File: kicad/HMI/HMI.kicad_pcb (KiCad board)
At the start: 2 copper layers, 45 parts, among them J2 SWD, J3 DEM 128128A TMH-PW-N, J4 RIBBON, SW1 SW_Push, SW10 SW_Push, SW11 SW_Push, SW12 SW_Push, SW13 SW_Push, SW14 SW_Push, SW15 SW_Push, SW16 SW_Push, SW17 SW_Push, SW18 SW_Push, SW19 SW_Push, SW2 SW_Push, SW20 SW_Push, SW3 SW_Push, SW4 SW_Push, SW5 SW_Push, SW6 SW_Push, SW7 SW_Push, SW8 SW_Push, SW9 SW_Push, U1 STM32L011K4Tx, X1 ASV-4.000MHZ-EJ-T

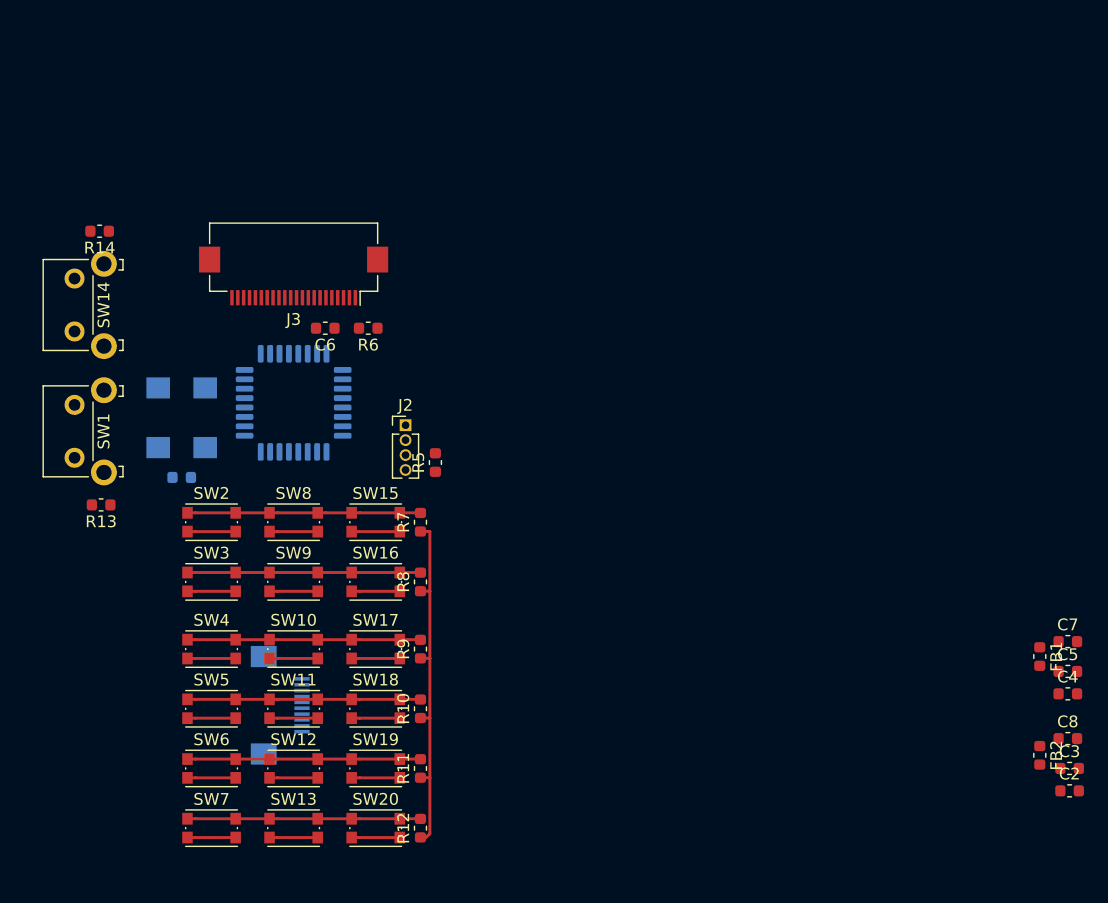
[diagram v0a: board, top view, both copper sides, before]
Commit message: HMI: added design of PCB -> plotted PDF -> plotted production output - Gerbers -> HMI is READY!!
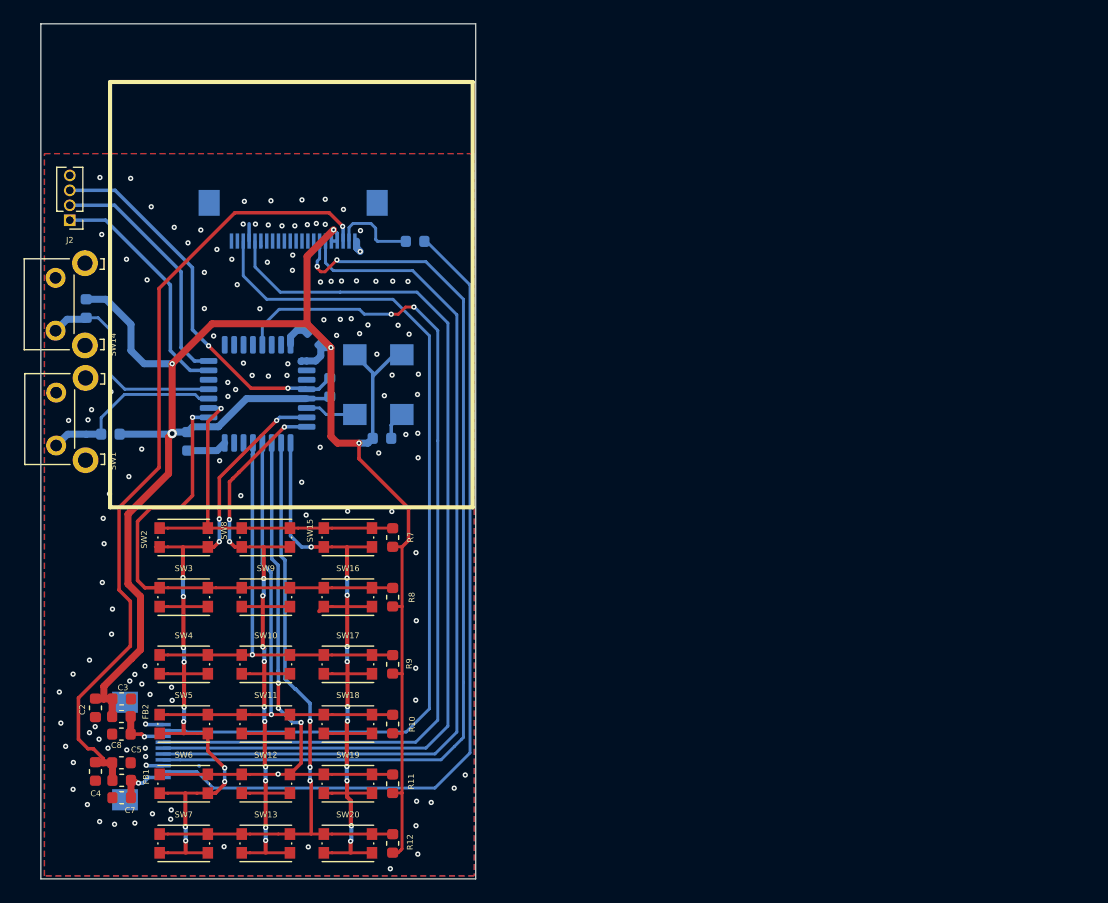
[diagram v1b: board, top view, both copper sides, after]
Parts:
- added C9: 1u, Capacitor_SMD:C_0603_1608Metric, B.Cu at (93.8, 67.5)
- C6, J3, R13, R14, R5, R6: moved to B.Cu
- moved C2 83.2 mm to (75.2, 99.0), turned to 270 degrees
- moved C4 83.0 mm to (75.2, 104.4), turned to 270 degrees
- moved C7 81.6 mm to (77.4, 106.6), turned to 180 degrees
- moved C5 80.9 mm to (77.4, 103.7)
- moved C3 80.9 mm to (77.4, 98.2)
- moved C8 80.5 mm to (77.4, 101.2), turned to 180 degrees
- moved FB1 78.8 mm to (77.4, 105.2), turned to 180 degrees
- moved FB2 78.2 mm to (77.4, 99.7), turned to 180 degrees
- moved J2 33.5 mm to (73.0, 57.5), turned to 180 degrees
- moved C1 17.4 mm to (99.6, 76.0), turned to 0 degrees
- moved X1 17.0 mm to (99.3, 71.5), turned to 270 degrees
- moved C6 15.2 mm to (83.1, 76.3), turned to 270 degrees
- moved J4 12.4 mm to (79.1, 102.7)
- moved R5 11.0 mm to (95.1, 71.7)
- moved R6 8.40 mm to (102.4, 59.3)
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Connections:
- J3 pad 16: GND -> SPI1_CS
- J3 pad 17: GND -> SPI1_SCK
- J3 pad 18: SPI1_MOSI -> +3V3
- J3 pad 19: GND -> +3V3
- J3 pad 2: Net-(J3-Pad2) -> GND
- J3 pad 20: TFT_RST -> +5V
- J3 pad 21: GND -> Net-(J3-Pad21)
- J3 pad 3: +5V -> TFT_RST
- J3 pad 4: +3V3 -> GND
- J3 pad 5: +3V3 -> SPI1_MOSI
- J3 pad 6: SPI1_SCK -> GND
- J3 pad 7: SPI1_CS -> GND
- R6 pad 2: Net-(J3-Pad2) -> Net-(J3-Pad21)
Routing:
- net +3V3: track 30.7 -> 159.1 mm, vias 0 -> 5
- net SPI1_CS: track 0.00 -> 80.4 mm, vias 0 -> 2
- net SPI1_MOSI: track 0.00 -> 79.9 mm
- net TFT_RST: track 0.00 -> 76.2 mm
- net SPI1_SCK: track 0.00 -> 76.1 mm
- net TX: track 0.00 -> 75.7 mm, vias 0 -> 2
- net TFT_LED: track 0.00 -> 73.2 mm
- net +5V: track 0.00 -> 68.2 mm, vias 0 -> 1
- net C1: track 24.6 -> 68.8 mm, vias 0 -> 13
- net C2: track 24.6 -> 65.8 mm, vias 0 -> 13
- net C3: track 24.6 -> 62.7 mm, vias 0 -> 11
- net R1: track 19.8 -> 54.2 mm, vias 0 -> 3
- net NRST: track 0.00 -> 32.6 mm, vias 0 -> 2
- net R2: track 19.8 -> 49.9 mm, vias 0 -> 4
- net R3: track 19.8 -> 44.0 mm, vias 0 -> 1
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- added copper zone on B.Cu, net GND
- added copper zone on F.Cu, net GND
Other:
- board outline added: 37 x 72.8 mm
- rule via_min_drill: 0.3 -> 0.2
- board text added: "1"
